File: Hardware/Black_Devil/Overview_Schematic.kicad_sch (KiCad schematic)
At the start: 11 parts, among them J15 Conn_01x03_Socket, J16 Klinke, J17 4mm, J18 Speakon, J19 Speakon, J20 4mm, J21 Klinke, T7 2x 45V 600VA, T8 2x 45V 600VA

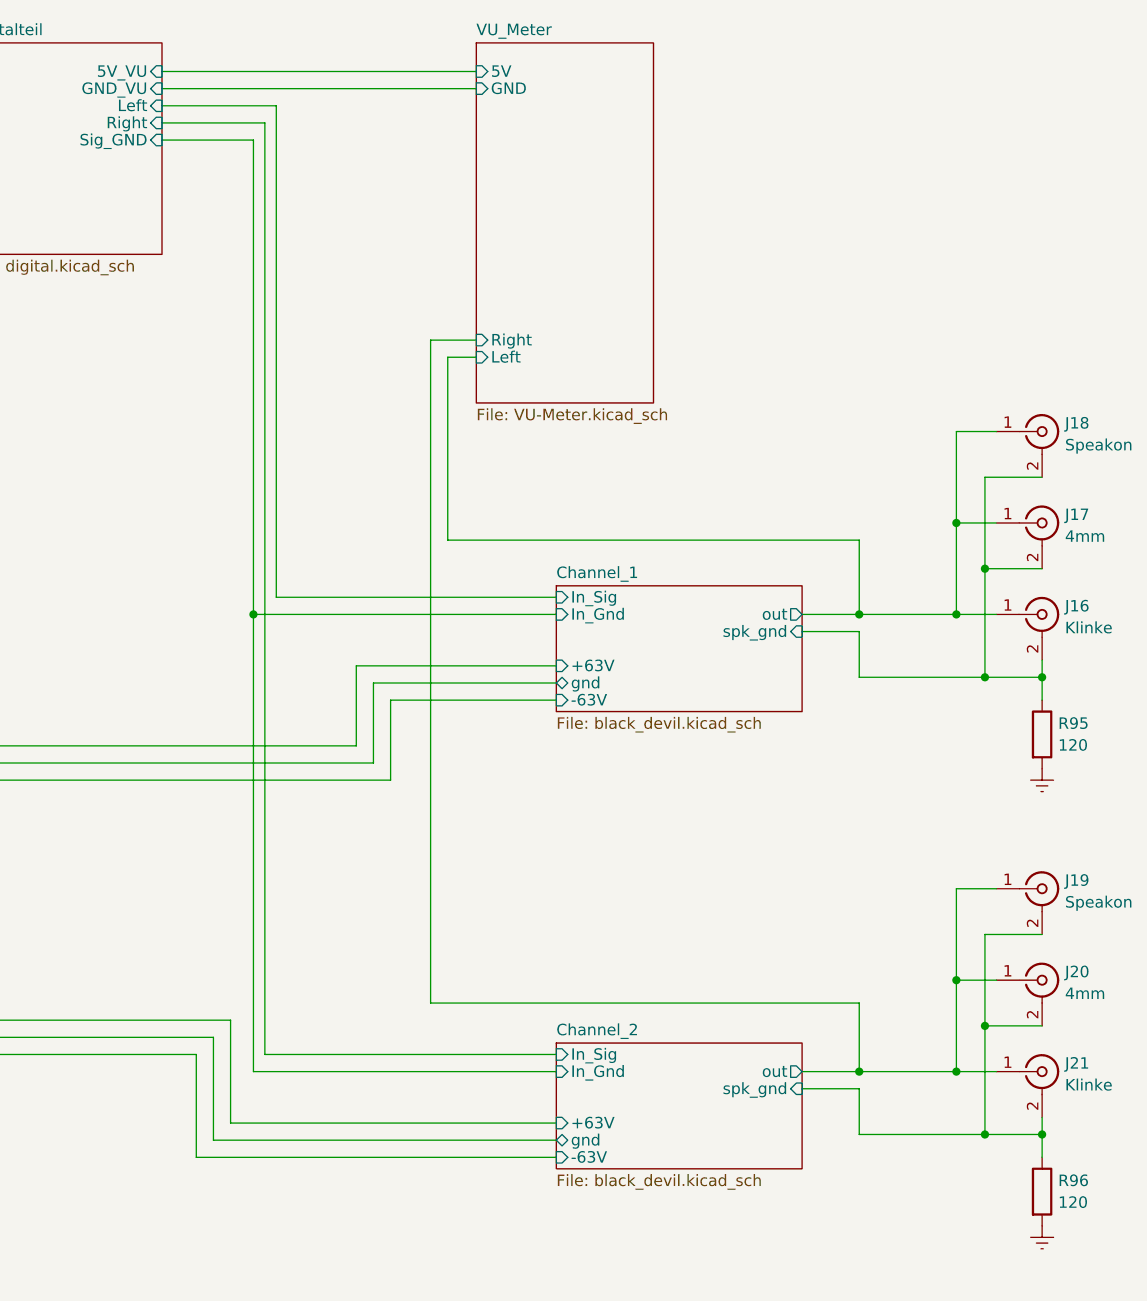
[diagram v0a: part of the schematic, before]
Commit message: Readme and Overview Update
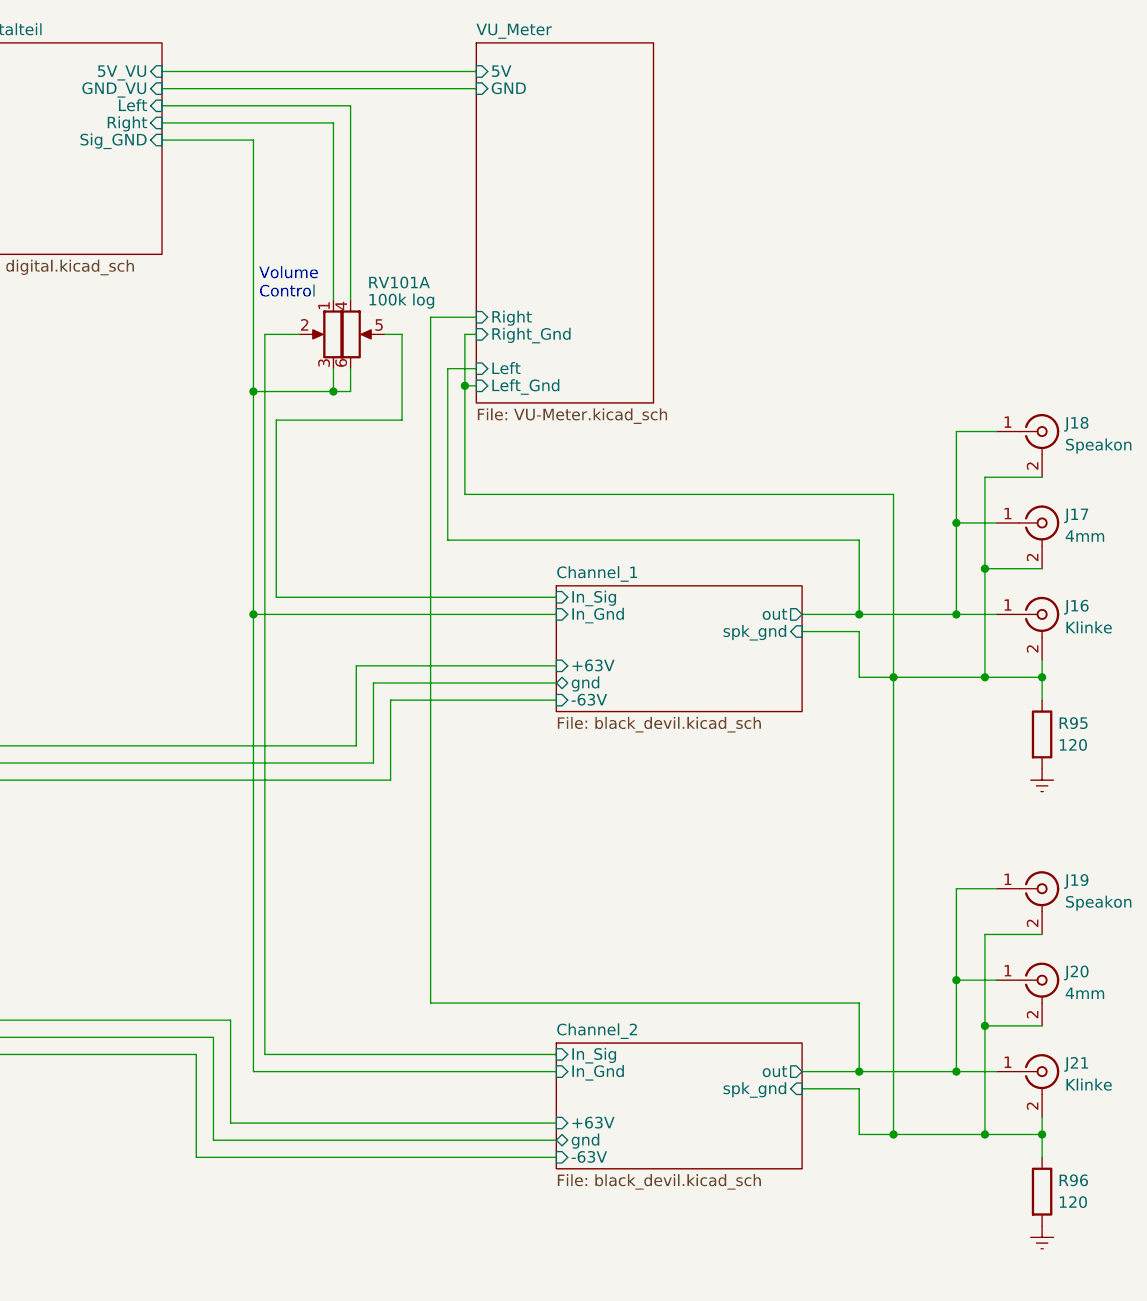
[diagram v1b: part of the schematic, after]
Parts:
- added RV101: 100k log, symbol Device:R_Potentiometer_Dual_Separate
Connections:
- net Channel_2/spk_gnd is gone; now on net Channel_1/spk_gnd: J19.2 (Ext), J20.2 (Ext), J21.2 (Ext), R96.1
- net Channel_1/In_Gnd: now also RV101.3, RV101.6
- net Channel_1/In_Sig: now also RV101.5
- net Channel_2/In_Sig: now also RV101.2
- new net Digitalteil/Left: RV101.4
- new net Digitalteil/Right: RV101.1
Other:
- sheet VU_Meter ports: added Left_Gnd, Right_Gnd; removed none
- note added: "Volume Control"
